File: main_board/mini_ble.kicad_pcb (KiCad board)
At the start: 4 copper layers, 74.8 x 31.2 mm, 127 parts, among them J1 FIX_M1.4, J2 FIX_M1.4, J4 FIX_M1.4, J7 FIX_M1.4, Q1 SI1013X, Q2 DMN1019USN, Q3 SI1013X, Q4 DMN1019USN, Q5 DMN1019USN, Q6 SI1013X, Q7 DMN1019USN, Q8 DMN1019USN, Q9 DMN1019USN, U1 MAX40200, U10 AT45DB081E, U11 USBC_Receptacle, U12 CON_SMARTCARD, U13 NC7SZ08P5X, U14 OLED_M01084, U15 LIS2HH12, U16 W25Q16, U17 SAMD21G18A-MU, U18 LM3670, U19 WHEEL_SRBE210200, U2 MIC5504, U3 TPS61220, U4 MAX40200, U5 LT1613, U6 MAX40200, U7 ATSAMD21E15B, U8 ATBTLC1000, U9 IP4234CZ6,125, Y1 32.768Khz, Y2 26Mhz

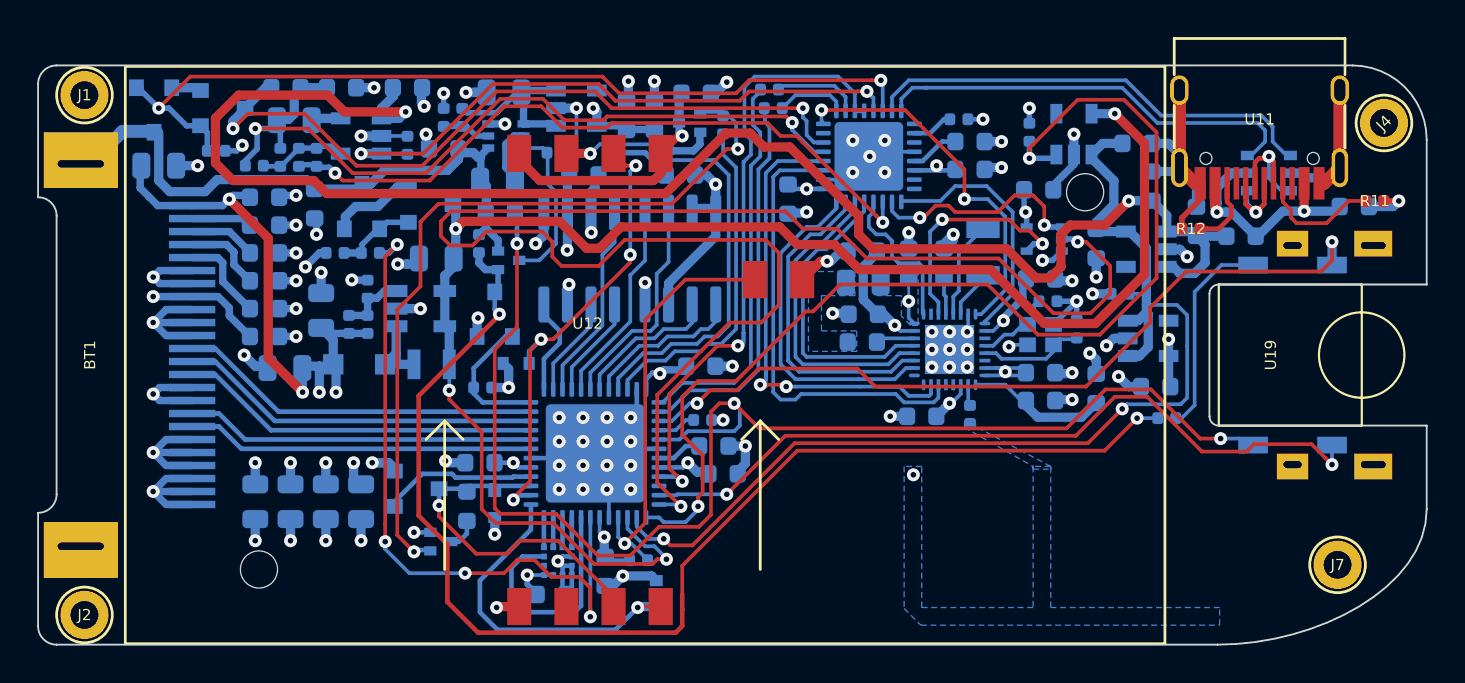
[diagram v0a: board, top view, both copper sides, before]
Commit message: updated
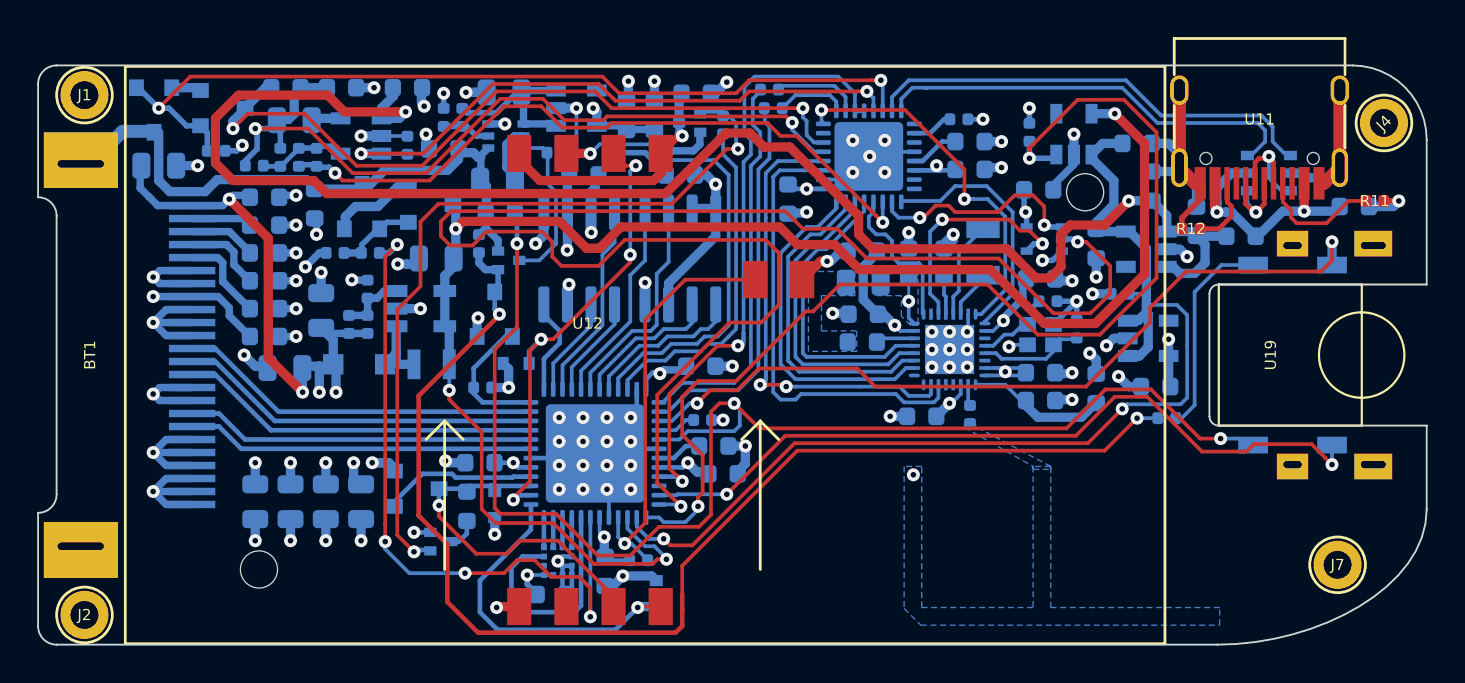
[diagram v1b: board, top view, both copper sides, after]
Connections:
- net /Main MCU & OLED/~RST renamed /Main MCU & OLED/~{RST}
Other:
- net class Default removed
